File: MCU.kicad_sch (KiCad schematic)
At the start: 23 parts, among them U7 STM32F405RGTx, Y1 16MHz

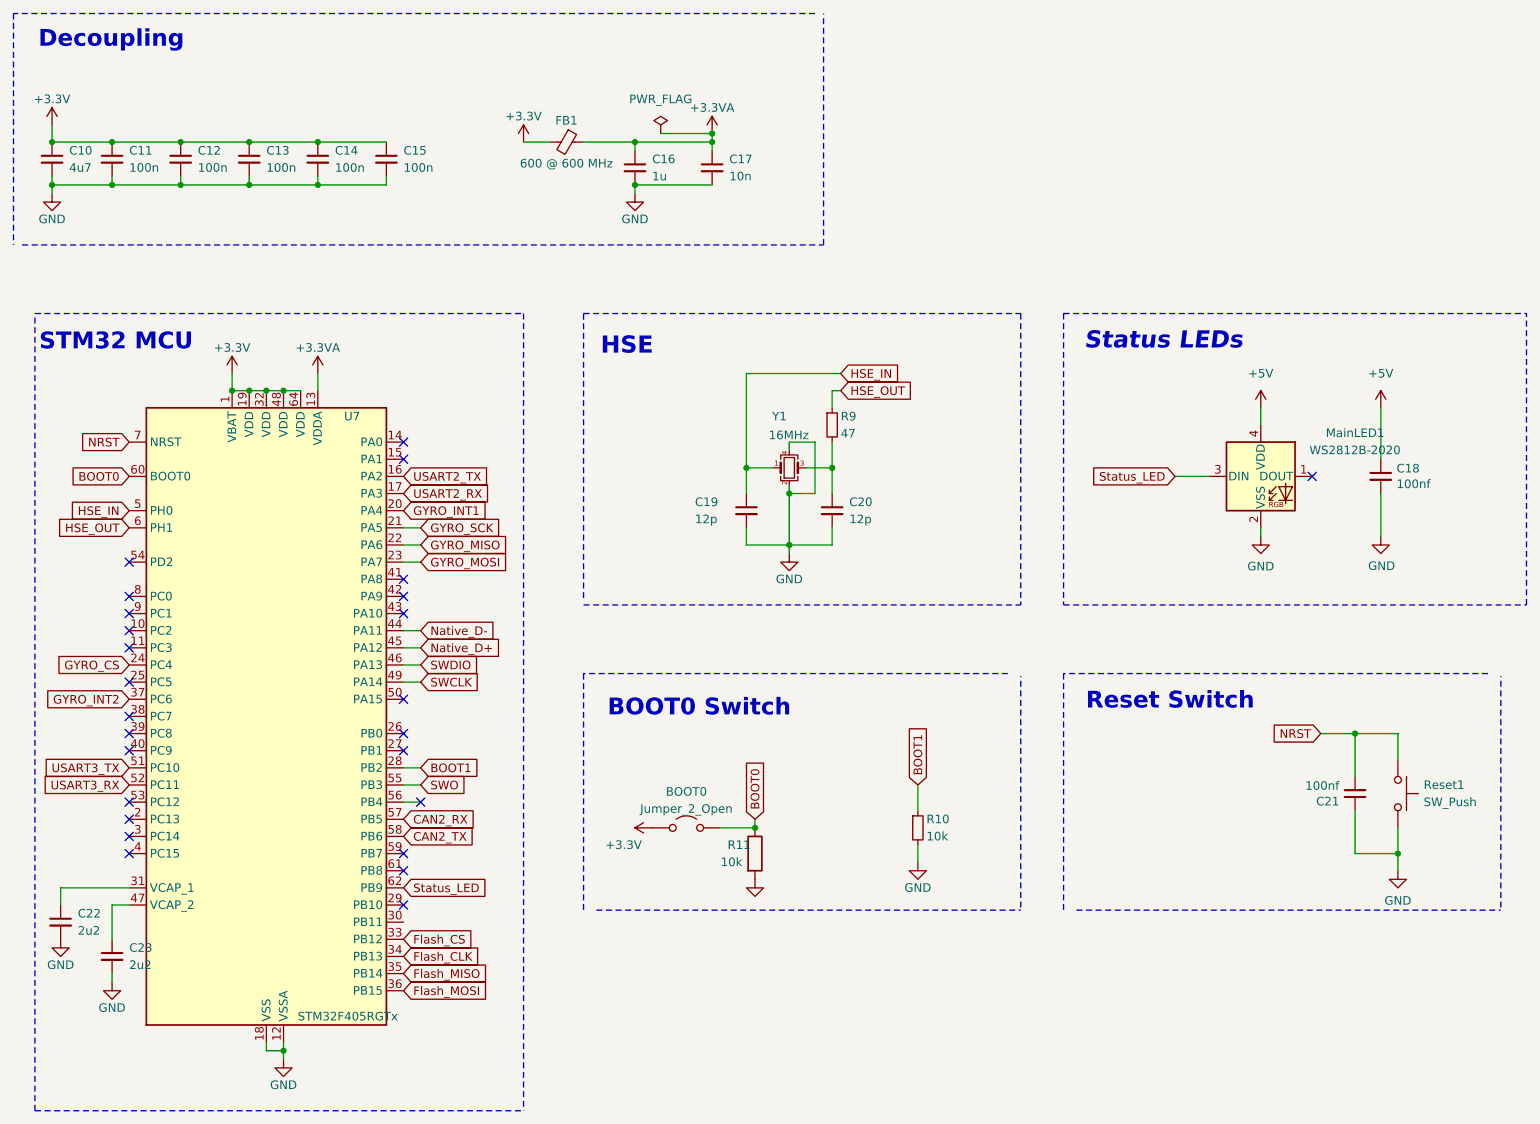
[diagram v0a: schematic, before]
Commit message: update
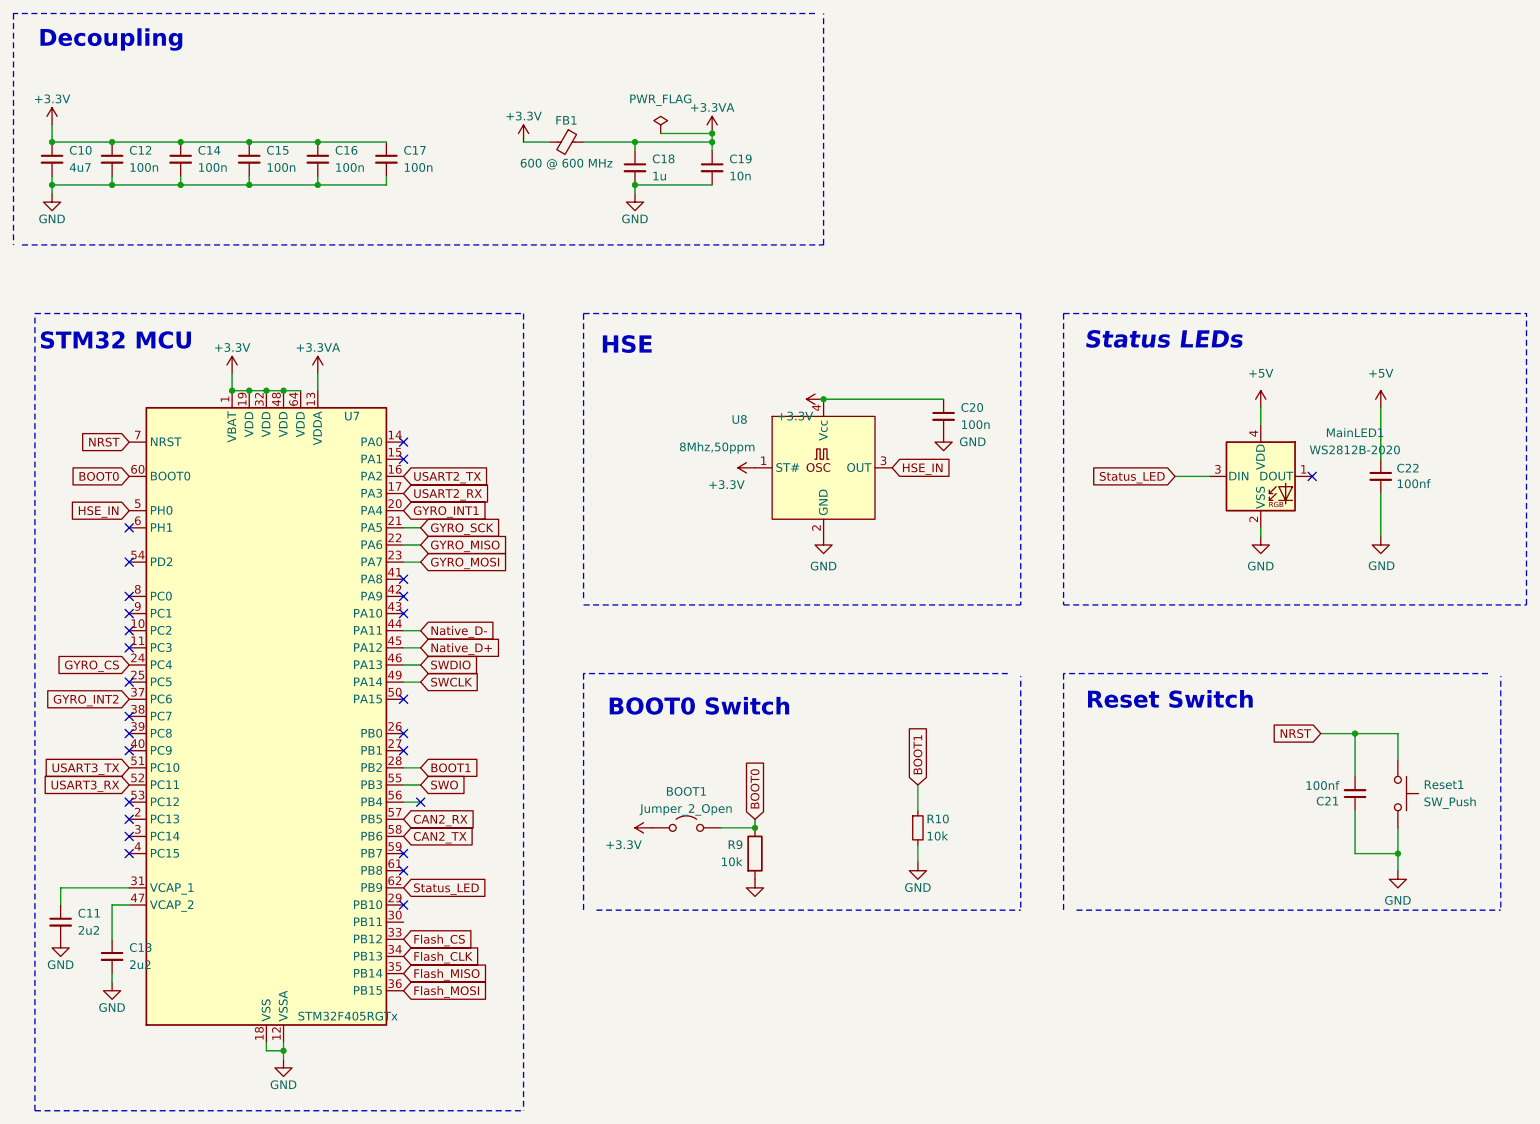
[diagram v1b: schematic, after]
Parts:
- removed C19: 12p, Capacitor_SMD:C_0402_1005Metric, symbol Device:C_Small
- removed R9: 47, Resistor_SMD:R_0402_1005Metric, symbol Device:R_Small
- removed Y1: 16MHz, Crystal:Crystal_SMD_3225-4Pin_3.2x2.5mm, symbol Device:Crystal_GND24_Small
- added U8: 8Mhz,50ppm, Oscillator:Oscillator_SMD_SeikoEpson_SG8002CE-4Pin_3.2x2.5mm, symbol bt_oscillator:OSC;12Mhz;50ppm;3v3;SG3225CAN
- C20: value 12p -> 100n; LCSC Part # C1547 -> C1525
- renumbered BOOT0 to BOOT1, C22 to C11, C11 to C12, C23 to C13, C12 to C14, C13 to C15, C14 to C16, C15 to C17, C16 to C18, C17 to C19, C18 to C22, R11 to R9
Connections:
- net +3.3V: now also C20.1, U8.1 (ST#), U8.4 (Vcc)
- net GND: now also U8.2 (GND)
- net HSE_IN: now also U8.3 (OUT)
- net HSE_OUT: no longer names the net of U7.6 (PH1)
- no-connect marks 26 -> 27

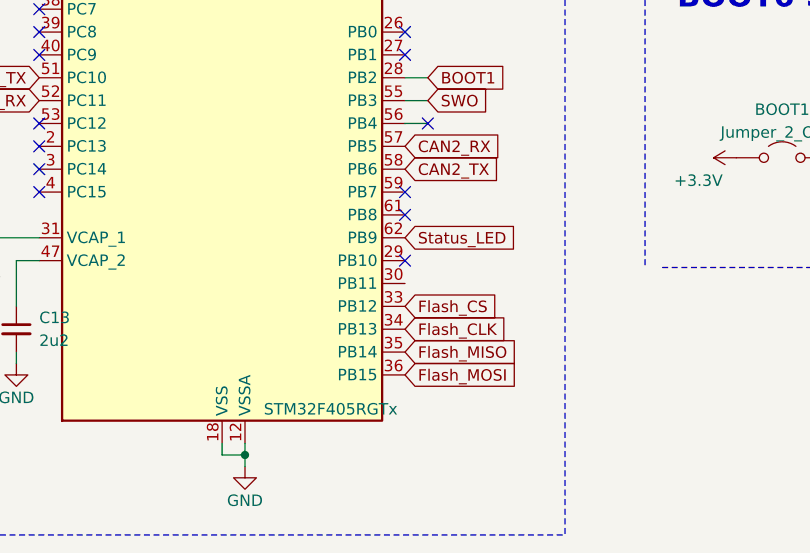
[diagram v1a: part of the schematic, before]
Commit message: update
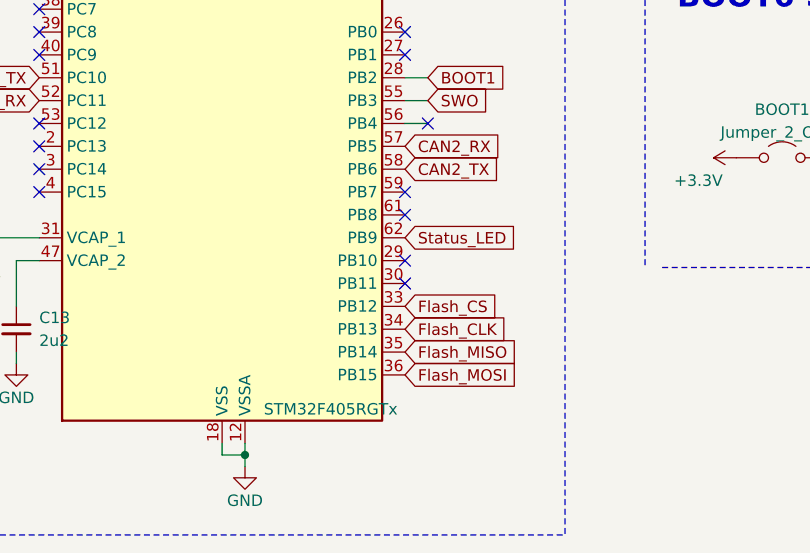
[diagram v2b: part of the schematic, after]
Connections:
- no-connect marks 27 -> 28
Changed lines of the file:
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@@
 	)
 	(no_connect
+		(at 102.87 162.56)
+	)
+	(no_connect
 		(at 102.87 160.02)
 	)
@@
 			)
 		)
-		(property "Description" "3V3 oscillator 12Mhz 50ppm"
+		(property "Description" "3V3 oscillator 8Mhz 50ppm"
 			(at 157.48 87.63 0)
 			(effects

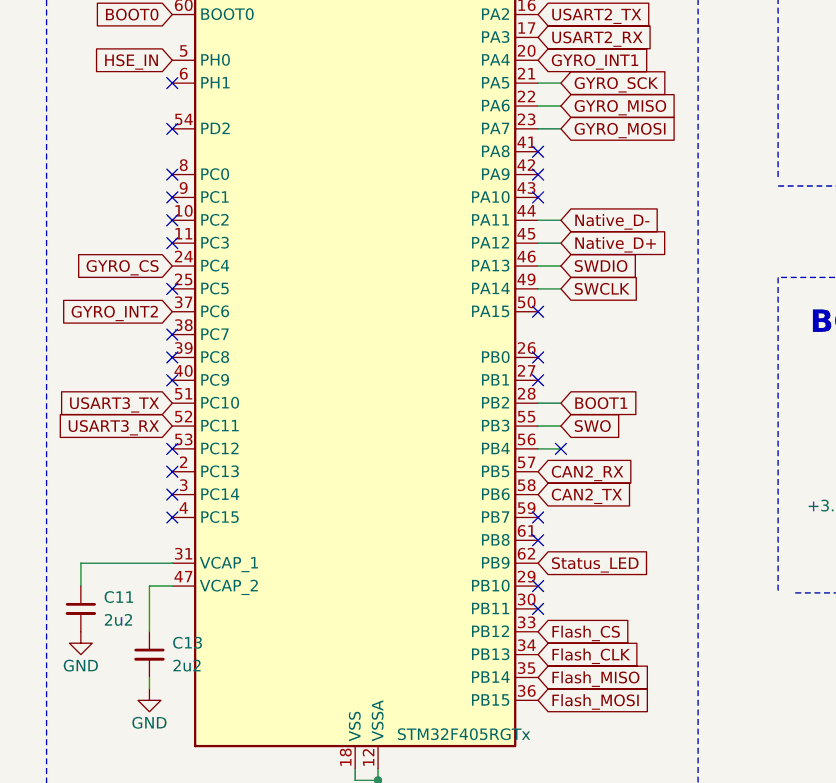
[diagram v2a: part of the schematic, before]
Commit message: update
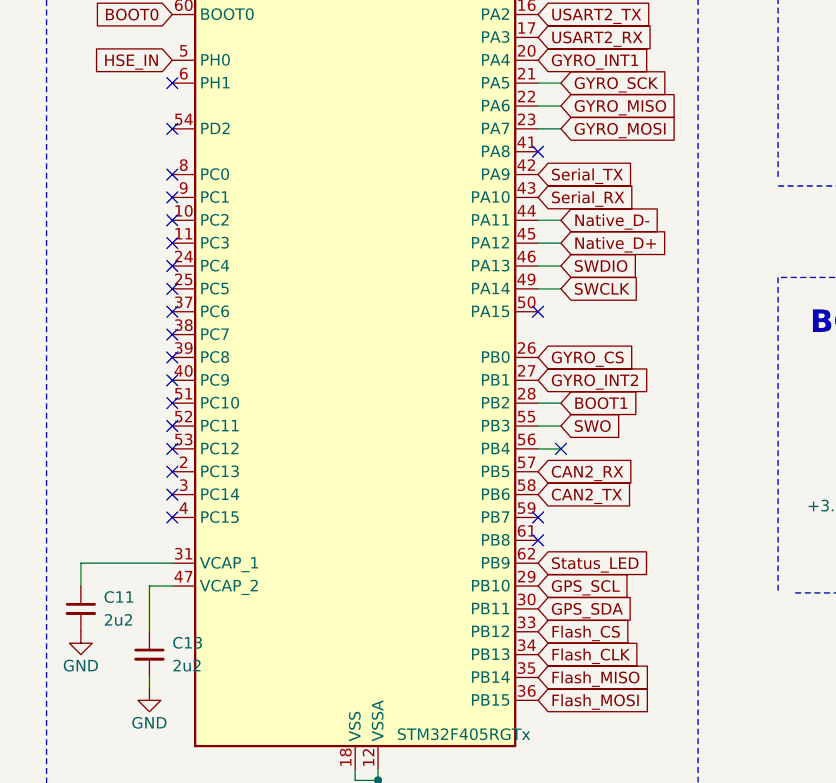
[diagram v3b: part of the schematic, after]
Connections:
- net GYRO_CS: now also U7.26 (PB0); no longer U7.24 (PC4)
- net GYRO_INT2: now also U7.27 (PB1); no longer U7.37 (PC6)
- net GPS_SCL: now reaches U7.29 (PB10)
- net GPS_SDA: now reaches U7.30 (PB11)
- net Serial_TX: now reaches U7.42 (PA9)
- net Serial_RX: now reaches U7.43 (PA10)
- net USART3_RX: no longer names the net of U7.52 (PC11)
- net USART3_TX: no longer names the net of U7.51 (PC10)
- no-connect marks 28 -> 26
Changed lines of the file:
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@@
 	)
 	(no_connect
-		(at 102.87 134.62)
+		(at 62.23 124.46)
 	)
 	(no_connect
@@
 	)
 	(no_connect
+		(at 62.23 129.54)
+	)
+	(no_connect
 		(at 62.23 147.32)
 	)
 	(no_connect
-		(at 102.87 162.56)
-	)
-	(no_connect
-		(at 102.87 160.02)
-	)
-	(no_connect
 		(at 62.23 116.84)
 	)
@@
 	)
 	(no_connect
-		(at 102.87 116.84)
-	)
-	(no_connect
-		(at 102.87 137.16)
-	)
-	(no_connect
 		(at 102.87 93.98)
 	)
@@
 	)
 	(no_connect
-		(at 102.87 114.3)
+		(at 62.23 142.24)
 	)
 	(no_connect
@@
 	(no_connect
 		(at 102.87 91.44)
+	)
+	(no_connect
+		(at 62.23 139.7)
 	)
 	(no_connect
@@
 		)
 	)
-	(global_label "GYRO_CS"
-		(shape input)
-		(at 62.23 124.46 180)
-		(effects
-			(font
-				(size 1.27 1.27)
-			)
-			(justify right)
-		)
-		(property "Intersheetrefs" "${INTERSHEET_REFS}"
-			(at 62.23 124.46 0)
-			(effects
-				(font
-					(size 1.27 1.27)
-				)
-				(hide yes)
-			)
-		)
-	)
 	(global_label "SWCLK"
 		(shape input)
@@
 		)
 	)
+	(global_label "GYRO_CS"
+		(shape input)
+		(at 102.87 134.62 0)
+		(effects
+			(font
+				(size 1.27 1.27)
+			)
+			(justify left)
+		)
+		(property "Intersheetrefs" "${INTERSHEET_REFS}"
+			(at 102.87 134.62 0)
+			(effects
+				(font
+					(size 1.27 1.27)
+				)
+				(hide yes)
+			)
+		)
+	)
 	(global_label "USART2_TX"
 		(shape input)
@@
 		)
 	)
-	(global_label "USART3_TX"
-		(shape input)
-		(at 62.23 139.7 180)
-		(effects
-			(font
-				(size 1.27 1.27)
-			)
-			(justify right)
-		)
-		(property "Intersheetrefs" "${INTERSHEET_REFS}"
-			(at 62.23 139.7 0)
-			(effects
-				(font
-					(size 1.27 1.27)
-				)
-				(hide yes)
-			)
-		)
-	)
 	(global_label "BOOT1"
 		(shape input)
@@
 		(property "Intersheetrefs" "${INTERSHEET_REFS}"
 			(at 105.41 139.7 0)
-			(effects
-				(font
-					(size 1.27 1.27)
-				)
-				(hide yes)
-			)
-		)
-	)
-	(global_label "USART3_RX"
-		(shape input)
-		(at 62.23 142.24 180)
-		(effects
-			(font
-				(size 1.27 1.27)
-			)
-			(justify right)
-		)
-		(property "Intersheetrefs" "${INTERSHEET_REFS}"
-			(at 62.23 142.24 0)
 			(effects
 				(font
@@
 		)
 	)
+	(global_label "GPS_SCL"
+		(shape input)
+		(at 102.87 160.02 0)
+		(fields_autoplaced yes)
+		(effects
+			(font
+				(size 1.27 1.27)
+			)
+			(justify left)
+		)
+		(property "Intersheetrefs" "${INTERSHEET_REFS}"
+			(at 114.0799 160.02 0)
+			(effects
+				(font
+					(size 1.27 1.27)
+				)
+				(justify left)
+				(hide yes)
+			)
+		)
+	)
 	(global_label "GYRO_MISO"
 		(shape input)
@@
 		)
 	)
+	(global_label "GYRO_INT2"
+		(shape input)
+		(at 102.87 137.16 0)
+		(effects
+			(font
+				(size 1.27 1.27)
+			)
+			(justify left)
+		)
+		(property "Intersheetrefs" "${INTERSHEET_REFS}"
+			(at 102.87 137.16 0)
+			(effects
+				(font
+					(size 1.27 1.27)
+				)
+				(hide yes)
+			)
+		)
+	)
+	(global_label "GPS_SDA"
+		(shape input)
+		(at 102.87 162.56 0)
+		(fields_autoplaced yes)
+		(effects
+			(font
+				(size 1.27 1.27)
+			)
+			(justify left)
+		)
+		(property "Intersheetrefs" "${INTERSHEET_REFS}"
+			(at 114.1404 162.56 0)
+			(effects
+				(font
+					(size 1.27 1.27)
+				)
+				(justify left)
+				(hide yes)
+			)
+		)
+	)
+	(global_label "Serial_RX"
+		(shape input)
+		(at 102.87 116.84 0)
+		(effects
+			(font
+				(size 1.27 1.27)
+			)
+			(justify left)
+		)
+		(property "Intersheetrefs" "${INTERSHEET_REFS}"
+			(at 102.87 116.84 0)
+			(effects
+				(font
+					(size 1.27 1.27)
+				)
+				(hide yes)
+			)
+		)
+	)
 	(global_label "Native_D+"
 		(shape input)
@@
 		)
 	)
+	(global_label "Serial_TX"
+		(shape input)
+		(at 102.87 114.3 0)
+		(effects
+			(font
+				(size 1.27 1.27)
+			)
+			(justify left)
+		)
+		(property "Intersheetrefs" "${INTERSHEET_REFS}"
+			(at 102.87 114.3 0)
+			(effects
+				(font
+					(size 1.27 1.27)
+				)
+				(hide yes)
+			)
+		)
+	)
 	(global_label "BOOT1"
 		(shape input)
@@
 			(effects
 				(font
-					(size 1.27 1.27)
-				)
-				(hide yes)
-			)
-		)
-	)
-	(global_label "GYRO_INT2"
-		(shape input)
-		(at 62.23 129.54 180)
-		(effects
-			(font
-				(size 1.27 1.27)
-			)
-			(justify right)
-		)
-		(property "Intersheetrefs" "${INTERSHEET_REFS}"
-			(at 62.23 129.54 0)
-			(effects
-				(font

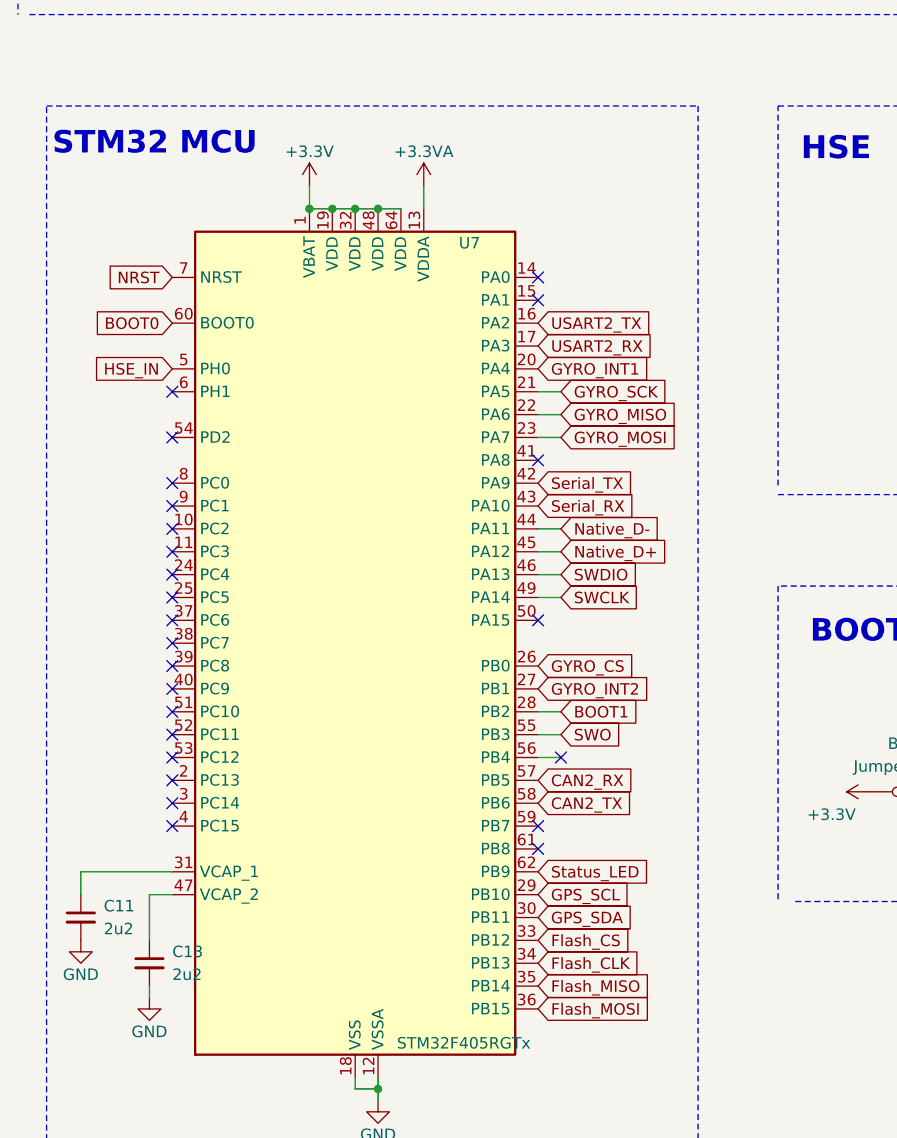
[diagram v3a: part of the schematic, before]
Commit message: update
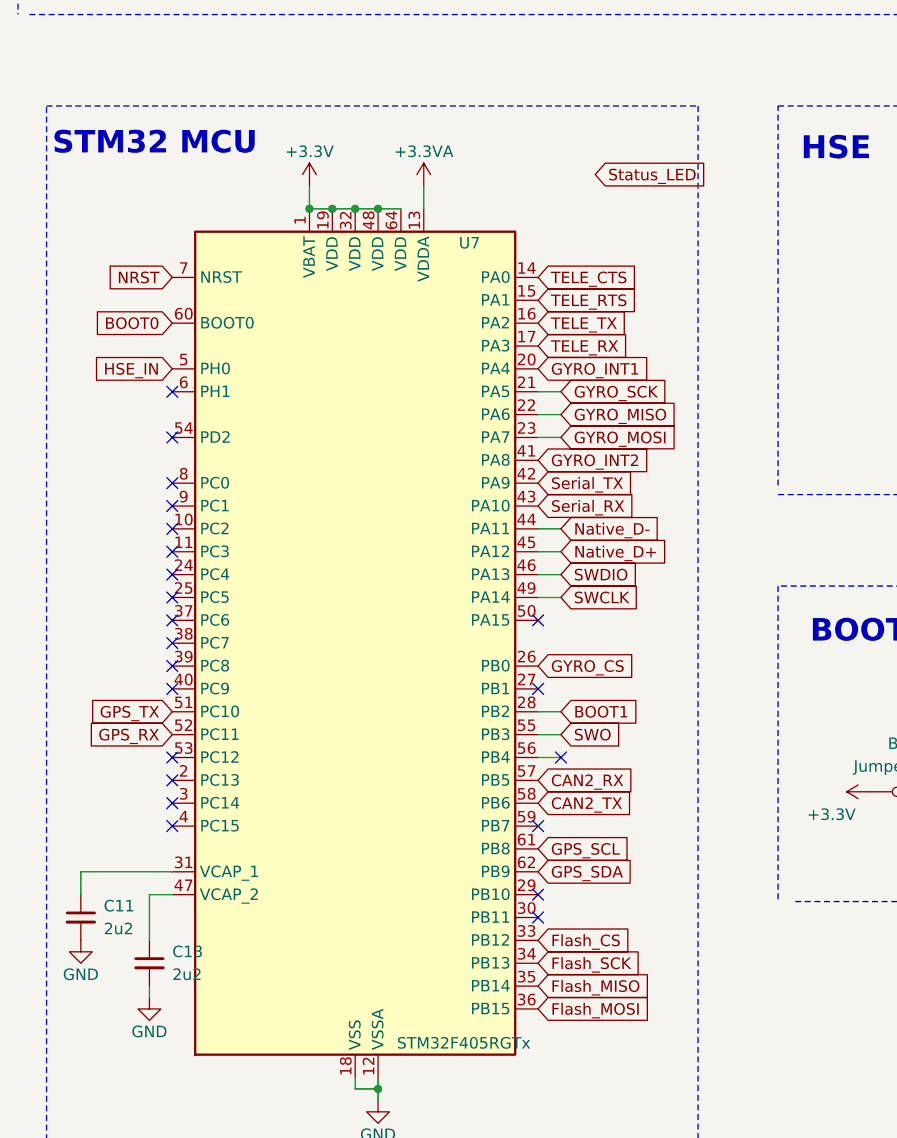
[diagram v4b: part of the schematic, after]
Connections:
- net GPS_SCL: now also U7.61 (PB8); no longer U7.29 (PB10)
- net GPS_SDA: now also U7.62 (PB9); no longer U7.30 (PB11)
- net GYRO_INT2: now also U7.41 (PA8); no longer U7.27 (PB1)
- net Status_LED: no longer U7.62 (PB9)
- net TELE_CTS: now reaches U7.14 (PA0)
- net TELE_RTS: now reaches U7.15 (PA1)
- net GPS_TX: now reaches U7.51 (PC10)
- net GPS_RX: now reaches U7.52 (PC11)
- net Flash_CLK renamed Flash_SCK
- net USART2_RX renamed TELE_RX
- net USART2_TX renamed TELE_TX
- no-connect marks 26 -> 23
